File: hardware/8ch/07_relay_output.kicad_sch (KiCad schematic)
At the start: 0 parts

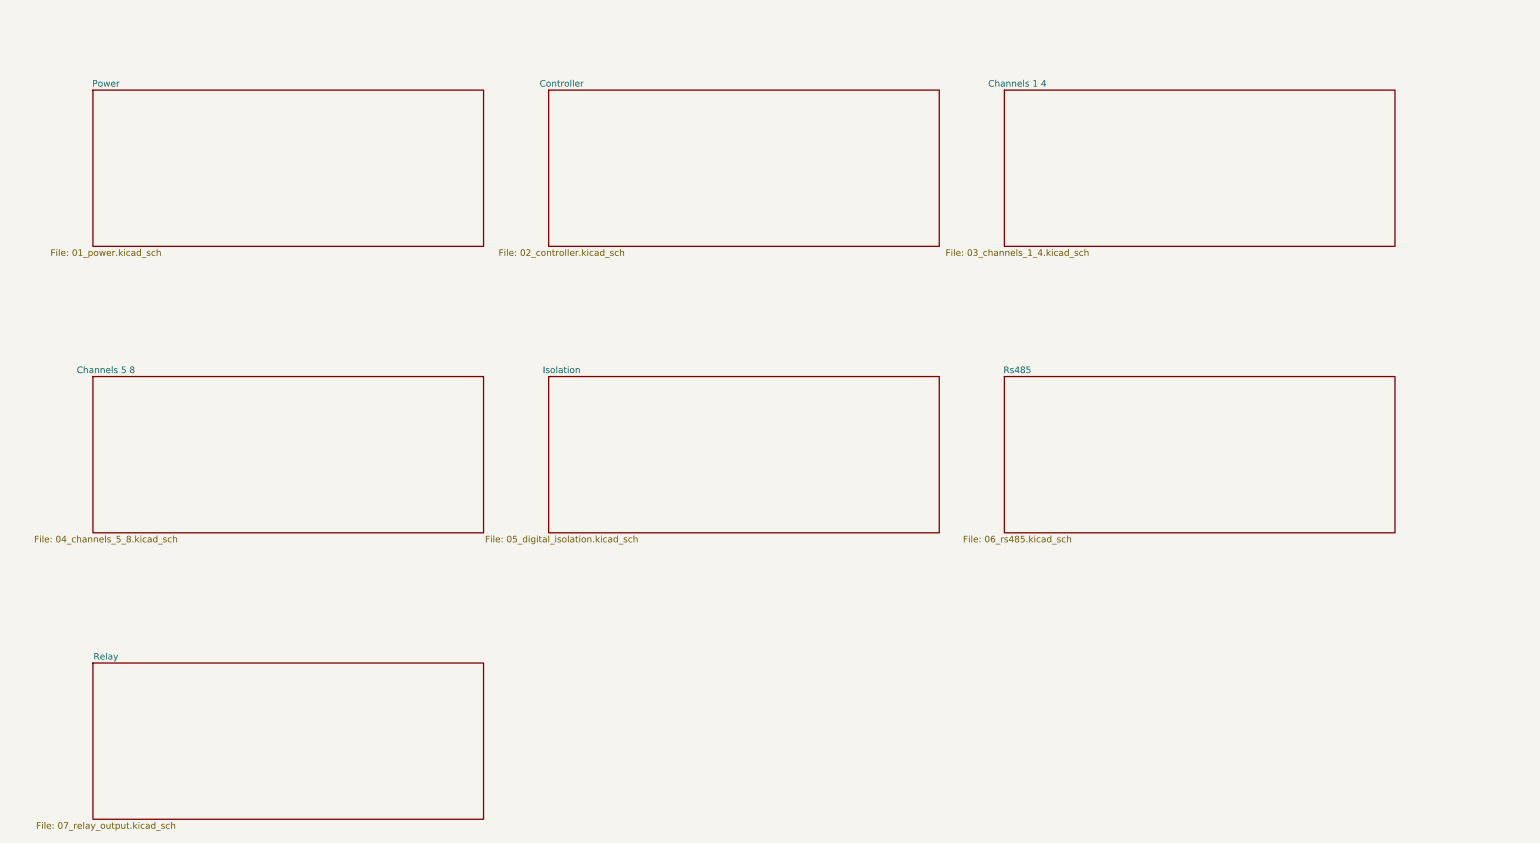
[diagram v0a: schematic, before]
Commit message: fix bugs
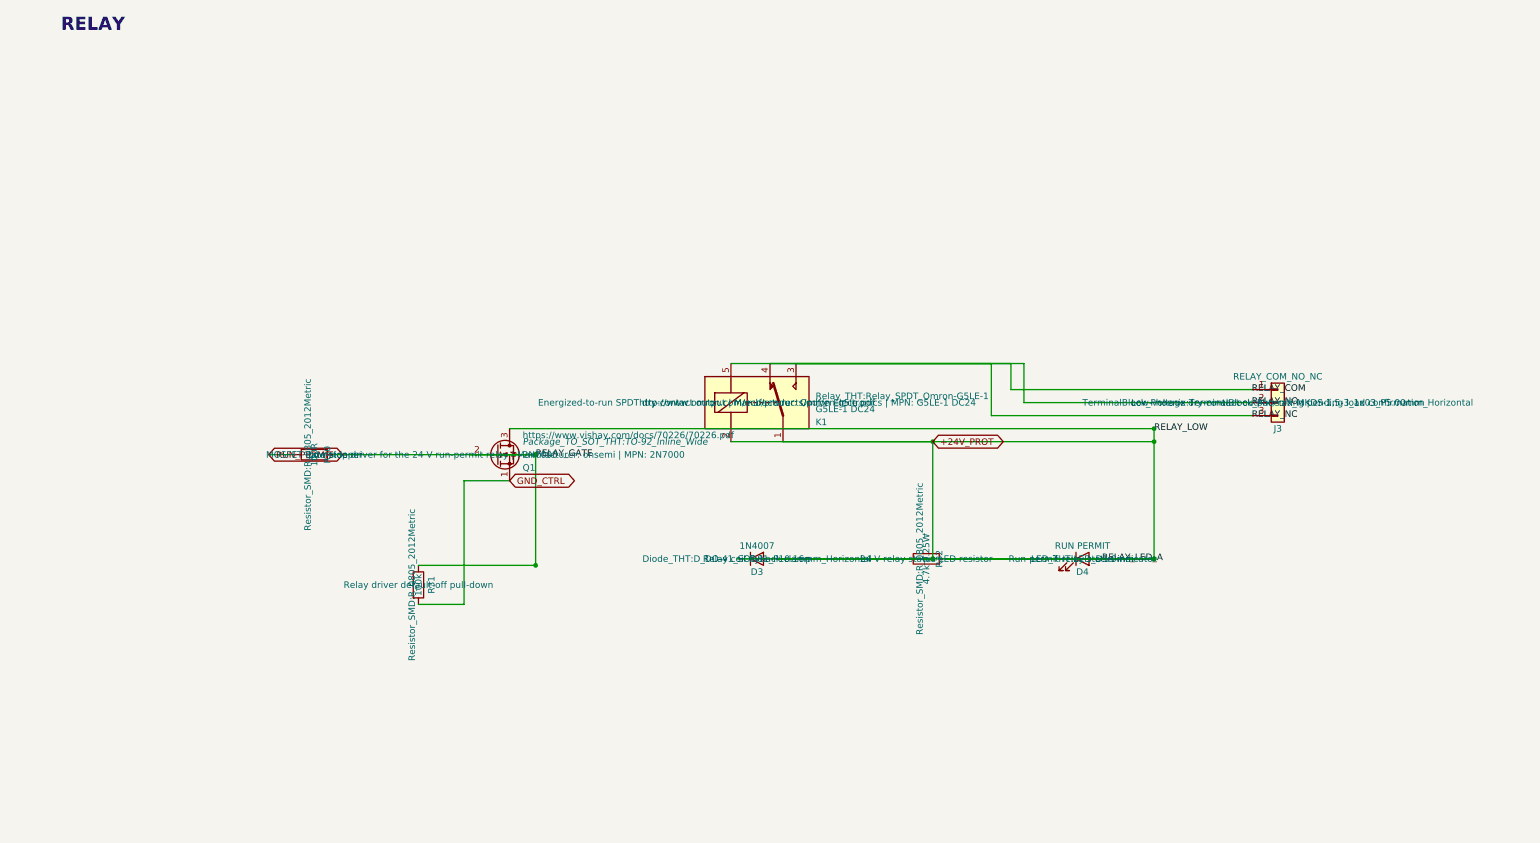
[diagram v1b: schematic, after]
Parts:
- added D3: 1N4007, Diode_THT:D_DO-41_SOD81_P10.16mm_Horizontal, symbol Device:D
- added D4: RUN PERMIT, LED_THT:LED_D3.0mm, symbol Device:LED
- added J3: RELAY_COM_NO_NC, TerminalBlock_Phoenix:TerminalBlock_Phoenix_MKDS-1,5-3_1x03_P5.00mm_Horizontal, symbol Connector_Generic:Conn_01x03
- added K1: G5LE-1 DC24, Relay_THT:Relay_SPDT_Omron-G5LE-1, symbol Relay:G5LE-1
- added Q1: 2N7000, Package_TO_SOT_THT:TO-92_Inline_Wide, symbol Transistor_FET:2N7000
- added R30: 100R, Resistor_SMD:R_0805_2012Metric, symbol Device:R
- added R31: 100k, Resistor_SMD:R_0805_2012Metric, symbol Device:R
- added R32: 4.7k 0.25W, Resistor_SMD:R_0805_2012Metric, symbol Device:R
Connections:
- new net +24V_PROT: D3.1 (K), D3.2 (A), D4.1 (K), D4.2 (A), K1.1, K1.2, Q1.3 (D), R32.1, R32.2
- new net GND_CTRL: Q1.1 (S), R31.2
- new net RELAY_COM: J3.1 (Pin_1), J3.2 (Pin_2), J3.3 (Pin_3), K1.3, K1.4, K1.5
- new net RELAY_GATE: Q1.2 (G), R30.2, R31.1
- new net RUN_PERMIT: R30.1
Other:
- removed sheet Channels 1 4
- removed sheet Channels 5 8
- removed sheet Controller
- removed sheet Isolation
- removed sheet Power
- removed sheet Relay
- removed sheet Rs485
- note added: "RELAY"
